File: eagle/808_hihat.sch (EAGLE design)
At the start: 101 parts, among them IC1 TL072P, IC3 TL071P, Q1 2N3904, Q10 2N3904, Q11 2N3904, Q12 2N3904, Q13 2N3906, Q14 2N3906, Q2 2N3904, Q3 2N3904, Q4 2N3904, Q5 2N3904, Q6 2N3904, Q7 2N3904, Q8 2N3904, Q9 2N3904

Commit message: 94pct ar
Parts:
- R130*, R140*, R173*: device TR808clone:R-EU_0207/5V -> TR808clone:R-EU_0207/7
- R145*, R162*: device TR808clone:R-EU_0207/7 -> TR808clone:R-EU_0207/5V
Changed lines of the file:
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@@
 <part name="V362" library="supply1" deviceset="GND" device=""/>
 <part name="V363" library="supply1" deviceset="GND" device=""/>
-<part name="R130*" library="TR808clone" deviceset="R-EU_" device="0207/5V" value="10K"/>
+<part name="R130*" library="TR808clone" deviceset="R-EU_" device="0207/7" value="10K"/>
 <part name="V364" library="supply1" deviceset="GND" device=""/>
 <part name="C60*" library="TR808clone" deviceset="CPOL-EU" device="E2.5-5" value="10/16"/>
@@
 <part name="R136*" library="TR808clone" deviceset="R-EU_" device="0207/5V" value="100R"/>
 <part name="R141*" library="TR808clone" deviceset="R-EU_" device="0207/5V" value="33K"/>
-<part name="R173*" library="TR808clone" deviceset="R-EU_" device="0207/5V" value="330K"/>
+<part name="R173*" library="TR808clone" deviceset="R-EU_" device="0207/7" value="330K"/>
 <part name="C63*" library="TR808clone" deviceset="CPOL-EU" device="E2.5-5" value=".47/50"/>
 <part name="V374" library="supply1" deviceset="GND" device=""/>
@@
 <part name="V375" library="supply1" deviceset="GND" device=""/>
 <part name="V376" library="supply1" deviceset="GND" device=""/>
-<part name="R145*" library="TR808clone" deviceset="R-EU_" device="0207/7" value="100R"/>
+<part name="R145*" library="TR808clone" deviceset="R-EU_" device="0207/5V" value="100R"/>
 <part name="R152*" library="TR808clone" deviceset="R-EU_" device="0207/5V" value="100R"/>
 <part name="R150*" library="TR808clone" deviceset="R-EU_" device="0207/5V" value="2M"/>
@@
 <part name="C74*" library="TR808clone" deviceset="C-EU" device="050-025X075" value="470p"/>
 <part name="R160*" library="TR808clone" deviceset="R-EU_" device="0207/5V" value="39K"/>
-<part name="R162*" library="TR808clone" deviceset="R-EU_" device="0207/7" value="33K"/>
+<part name="R162*" library="TR808clone" deviceset="R-EU_" device="0207/5V" value="33K"/>
 <part name="R158*" library="TR808clone" deviceset="R-EU_" device="0207/5V" value="47K"/>
 <part name="R157*" library="TR808clone" deviceset="R-EU_" device="0207/5V" value="47K"/>
@@
 <part name="R172*" library="TR808clone" deviceset="R-EU_" device="0207/7" value="1K"/>
 <part name="R132*" library="TR808clone" deviceset="R-EU_" device="0207/5V" value="100K"/>
-<part name="R140*" library="TR808clone" deviceset="R-EU_" device="0207/5V" value="33K"/>
+<part name="R140*" library="TR808clone" deviceset="R-EU_" device="0207/7" value="33K"/>
 <part name="R156*" library="TR808clone" deviceset="R-EU_" device="0207/7" value="22K"/>
 <part name="R154*" library="TR808clone" deviceset="R-EU_" device="0207/5V" value="22K"/>

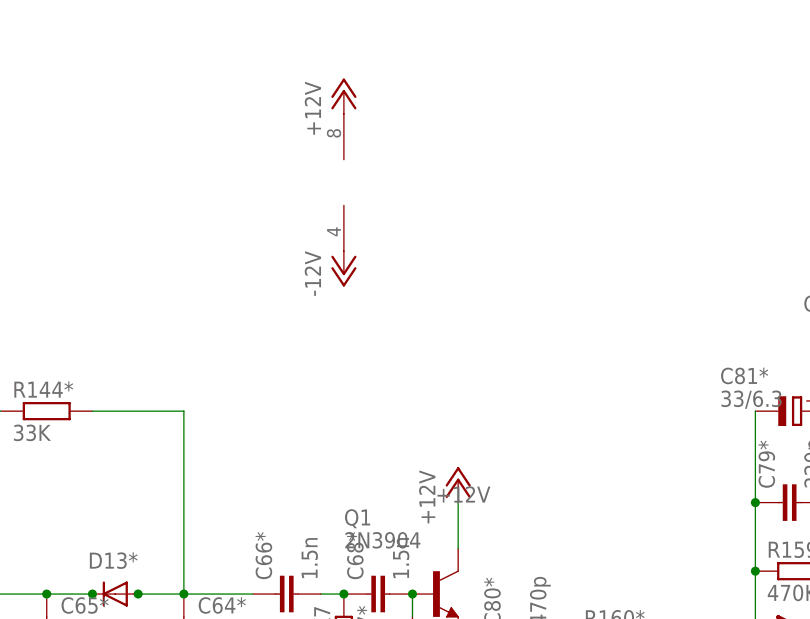
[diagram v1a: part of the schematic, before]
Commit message: 94pct6 ar
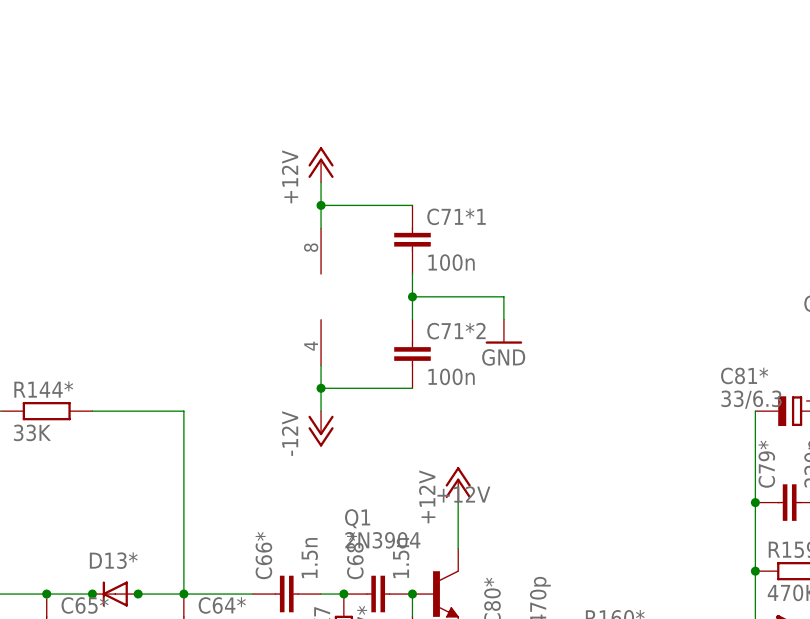
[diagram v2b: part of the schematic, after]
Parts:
- added C71*1, C71*2: 100n, TR808clone:C-EU3MM_PITCH
- C64*, C66*, C72*, C73*: device TR808clone:C-EU3.5MM_PITCH -> TR808clone:C-EU050-024X044
- C81*: device TR808clone:CPOL-EUE2-5 -> TR808clone:CPOL-EUE3.5-8
- R135*, R155*, R158*, R162*: device TR808clone:R-EU_0207/5V -> TR808clone:R-EU_0207/7
- R136*: device TR808clone:R-EU_0207/5V -> TR808clone:R-EU_0207/2V
- R156*, R172*: device TR808clone:R-EU_0207/7 -> TR808clone:R-EU_0207/5V
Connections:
- net +12V: now also C71*1.1
- net -12V: now also C71*2.2
- net GND: now also C71*1.2, C71*2.1
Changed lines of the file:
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@@
 <part name="R133*" library="TR808clone" deviceset="R-EU_" device="0207/7" value="10K"/>
 <part name="R134*" library="TR808clone" deviceset="R-EU_" device="0207/7" value="100K"/>
-<part name="R135*" library="TR808clone" deviceset="R-EU_" device="0207/5V" value="10K"/>
+<part name="R135*" library="TR808clone" deviceset="R-EU_" device="0207/7" value="10K"/>
 <part name="R137*" library="TR808clone" deviceset="R-EU_" device="0207/5V" value="470R"/>
 <part name="C62*" library="TR808clone" deviceset="CPOL-EU" device="E2.5-5" value=".47/50"/>
@@
 <part name="R143*" library="TR808clone" deviceset="R-EU_" device="0207/5V" value="33K"/>
 <part name="V371" library="supply1" deviceset="GND" device=""/>
-<part name="R136*" library="TR808clone" deviceset="R-EU_" device="0207/5V" value="100R"/>
+<part name="R136*" library="TR808clone" deviceset="R-EU_" device="0207/2V" value="100R"/>
 <part name="R141*" library="TR808clone" deviceset="R-EU_" device="0207/5V" value="33K"/>
 <part name="R173*" library="TR808clone" deviceset="R-EU_" device="0207/7" value="330K"/>
@@
 <part name="C65*" library="TR808clone" deviceset="C-EU" device="3.5MM_PITCH" value="1.5n"/>
 <part name="C70*" library="TR808clone" deviceset="C-EU" device="3.5MM_PITCH" value="1.5n"/>
-<part name="C64*" library="TR808clone" deviceset="C-EU" device="3.5MM_PITCH" value="1.5n"/>
+<part name="C64*" library="TR808clone" deviceset="C-EU" device="050-024X044" value="1.5n"/>
 <part name="C69*" library="TR808clone" deviceset="C-EU" device="3.5MM_PITCH" value="1.5n"/>
 <part name="V379" library="supply1" deviceset="GND" device=""/>
@@
 <part name="V381" library="supply1" deviceset="GND" device=""/>
 <part name="V382" library="supply1" deviceset="GND" device=""/>
-<part name="C66*" library="TR808clone" deviceset="C-EU" device="3.5MM_PITCH" value="1.5n"/>
-<part name="C72*" library="TR808clone" deviceset="C-EU" device="3.5MM_PITCH" value="1n"/>
+<part name="C66*" library="TR808clone" deviceset="C-EU" device="050-024X044" value="1.5n"/>
+<part name="C72*" library="TR808clone" deviceset="C-EU" device="050-024X044" value="1n"/>
 <part name="C68*" library="TR808clone" deviceset="C-EU" device="050-024X044" value="1.5n"/>
-<part name="C73*" library="TR808clone" deviceset="C-EU" device="3.5MM_PITCH" value="1n"/>
+<part name="C73*" library="TR808clone" deviceset="C-EU" device="050-024X044" value="1n"/>
 <part name="R147*" library="TR808clone" deviceset="R-EU_" device="0207/7" value="2K7"/>
 <part name="R153*" library="rcl" deviceset="R-US_" device="0207/5V" value="2K7"/>
 <part name="R146*" library="TR808clone" deviceset="R-EU_" device="0207/7" value="68K"/>
-<part name="R155*" library="TR808clone" deviceset="R-EU_" device="0207/5V" value="68K"/>
+<part name="R155*" library="TR808clone" deviceset="R-EU_" device="0207/7" value="68K"/>
 <part name="V383" library="supply1" deviceset="GND" device=""/>
 <part name="V384" library="supply1" deviceset="GND" device=""/>
@@
 <part name="C74*" library="TR808clone" deviceset="C-EU" device="050-025X075" value="470p"/>
 <part name="R160*" library="TR808clone" deviceset="R-EU_" device="0207/5V" value="39K"/>
-<part name="R162*" library="TR808clone" deviceset="R-EU_" device="0207/5V" value="33K"/>
-<part name="R158*" library="TR808clone" deviceset="R-EU_" device="0207/5V" value="47K"/>
+<part name="R162*" library="TR808clone" deviceset="R-EU_" device="0207/7" value="33K"/>
+<part name="R158*" library="TR808clone" deviceset="R-EU_" device="0207/7" value="47K"/>
 <part name="R157*" library="TR808clone" deviceset="R-EU_" device="0207/5V" value="47K"/>
 <part name="V389" library="supply1" deviceset="GND" device=""/>
 <part name="V390" library="supply1" deviceset="GND" device=""/>
 <part name="R159*" library="TR808clone" deviceset="R-EU_" device="0207/2V" value="470K"/>
-<part name="C81*" library="TR808clone" deviceset="CPOL-EU" device="E2-5" value="33/6.3"/>
+<part name="C81*" library="TR808clone" deviceset="CPOL-EU" device="E3.5-8" value="33/6.3"/>
 <part name="C79*" library="TR808clone" deviceset="C-EU" device="025-025X050" value="220p"/>
 <part name="R169*" library="TR808clone" deviceset="R-EU_" device="0207/7" value="1K"/>
@@
 <part name="C83*" library="TR808clone" deviceset="CPOL-EU" device="E2-5" value="33/6.3"/>
 <part name="C82*" library="TR808clone" deviceset="C-EU" device="025-025X050" value="220p"/>
-<part name="R172*" library="TR808clone" deviceset="R-EU_" device="0207/7" value="1K"/>
+<part name="R172*" library="TR808clone" deviceset="R-EU_" device="0207/5V" value="1K"/>
 <part name="R132*" library="TR808clone" deviceset="R-EU_" device="0207/5V" value="100K"/>
 <part name="R140*" library="TR808clone" deviceset="R-EU_" device="0207/7" value="33K"/>
-<part name="R156*" library="TR808clone" deviceset="R-EU_" device="0207/7" value="22K"/>
+<part name="R156*" library="TR808clone" deviceset="R-EU_" device="0207/5V" value="22K"/>
 <part name="R154*" library="TR808clone" deviceset="R-EU_" device="0207/5V" value="22K"/>
 <part name="R144*" library="TR808clone" deviceset="R-EU_" device="0207/5V" value="33K"/>
@@
 <part name="P+13" library="supply1" deviceset="+12V" device=""/>
 <part name="P-6" library="supply1" deviceset="-12V" device=""/>
+<part name="C71*1" library="TR808clone" deviceset="C-EU" device="3MM_PITCH" value="100n"/>
+<part name="C71*2" library="TR808clone" deviceset="C-EU" device="3MM_PITCH" value="100n"/>
+<part name="V5" library="supply1" deviceset="GND" device=""/>
 </parts>
 <sheets>
@@
 <instance part="Q13" gate="G$1" x="-50.8" y="93.98"/>
 <instance part="Q14" gate="G$1" x="-48.26" y="5.08"/>
-<instance part="IC1" gate="P" x="93.98" y="101.6"/>
-<instance part="P+5" gate="1" x="93.98" y="111.76"/>
-<instance part="P-5" gate="1" x="93.98" y="91.44"/>
+<instance part="IC1" gate="P" x="91.44" y="88.9"/>
+<instance part="P+5" gate="1" x="91.44" y="104.14"/>
+<instance part="P-5" gate="1" x="91.44" y="73.66"/>
 <instance part="IC3" gate="A" x="27.94" y="-30.48" rot="MR180"/>
 <instance part="P+13" gate="1" x="33.02" y="-38.1"/>
 <instance part="P-6" gate="1" x="22.86" y="-22.86"/>
+<instance part="C71*1" gate="G$1" x="101.6" y="96.52"/>
+<instance part="C71*2" gate="G$1" x="101.6" y="83.82"/>
+<instance part="V5" gate="1" x="111.76" y="83.82"/>
 </instances>
 <busses>
@@
 <pinref part="Q11" gate="G1" pin="E"/>
 </segment>
+<segment>
+<pinref part="V5" gate="1" pin="GND"/>
+<wire x1="111.76" y1="86.36" x2="111.76" y2="88.9" width="0.1524" layer="91"/>
+<pinref part="C71*2" gate="G$1" pin="1"/>
+<pinref part="C71*1" gate="G$1" pin="2"/>
+<wire x1="101.6" y1="86.36" x2="101.6" y2="88.9" width="0.1524" layer="91"/>
+<wire x1="101.6" y1="88.9" x2="101.6" y2="91.44" width="0.1524" layer="91"/>
+<wire x1="111.76" y1="88.9" x2="101.6" y2="88.9" width="0.1524" layer="91"/>
+<junction x="101.6" y="88.9"/>
+</segment>
 </net>
 <net name="N$219" class="0">
@@
 <pinref part="IC1" gate="P" pin="V+"/>
 <pinref part="P+5" gate="1" pin="+12V"/>
+<wire x1="91.44" y1="96.52" x2="91.44" y2="99.06" width="0.1524" layer="91"/>
+<pinref part="C71*1" gate="G$1" pin="1"/>
+<wire x1="91.44" y1="99.06" x2="91.44" y2="101.6" width="0.1524" layer="91"/>
+<wire x1="101.6" y1="99.06" x2="91.44" y2="99.06" width="0.1524" layer="91"/>
+<junction x="91.44" y="99.06"/>
 </segment>
 <segment>
@@
 <pinref part="IC1" gate="P" pin="V-"/>
 <pinref part="P-5" gate="1" pin="-12V"/>
-</segment>
-<segment>
+<wire x1="91.44" y1="76.2" x2="91.44" y2="78.74" width="0.1524" layer="91"/>
+<pinref part="C71*2" gate="G$1" pin="2"/>
+<wire x1="91.44" y1="78.74" x2="91.44" y2="81.28" width="0.1524" layer="91"/>
+<wire x1="101.6" y1="78.74" x2="91.44" y2="78.74" width="0.1524" layer="91"/>
+<junction x="91.44" y="78.74"/>
+</segment>
+<segment>

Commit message: rotated output amp looks promising
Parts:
- C68*: device TR808clone:C-EU050-024X044 -> TR808clone:C-EU050-025X075
- C69*, C80*: device TR808clone:C-EU3.5MM_PITCH -> TR808clone:C-EU050-024X044
- C71*1: device TR808clone:C-EU3MM_PITCH -> TR808clone:C-EU050-024X044
- R136*, R58*1: device TR808clone:R-EU_0207/2V -> TR808clone:R-EU_0207/5V
- R142*: device TR808clone:R-EU_0207/7 -> TR808clone:R-EU_0207/5V
- R147*: device TR808clone:R-EU_0207/7 -> TR808clone:R-EU_0309/10
- R156*, R157*, R160*: device TR808clone:R-EU_0207/5V -> TR808clone:R-EU_0207/7
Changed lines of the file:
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@@
 <part name="R143*" library="TR808clone" deviceset="R-EU_" device="0207/5V" value="33K"/>
 <part name="V371" library="supply1" deviceset="GND" device=""/>
-<part name="R136*" library="TR808clone" deviceset="R-EU_" device="0207/2V" value="100R"/>
+<part name="R136*" library="TR808clone" deviceset="R-EU_" device="0207/5V" value="100R"/>
 <part name="R141*" library="TR808clone" deviceset="R-EU_" device="0207/5V" value="33K"/>
 <part name="R173*" library="TR808clone" deviceset="R-EU_" device="0207/7" value="330K"/>
@@
 <part name="C70*" library="TR808clone" deviceset="C-EU" device="3.5MM_PITCH" value="1.5n"/>
 <part name="C64*" library="TR808clone" deviceset="C-EU" device="050-024X044" value="1.5n"/>
-<part name="C69*" library="TR808clone" deviceset="C-EU" device="3.5MM_PITCH" value="1.5n"/>
+<part name="C69*" library="TR808clone" deviceset="C-EU" device="050-024X044" value="1.5n"/>
 <part name="V379" library="supply1" deviceset="GND" device=""/>
 <part name="V380" library="supply1" deviceset="GND" device=""/>
@@
 <part name="C66*" library="TR808clone" deviceset="C-EU" device="050-024X044" value="1.5n"/>
 <part name="C72*" library="TR808clone" deviceset="C-EU" device="050-024X044" value="1n"/>
-<part name="C68*" library="TR808clone" deviceset="C-EU" device="050-024X044" value="1.5n"/>
+<part name="C68*" library="TR808clone" deviceset="C-EU" device="050-025X075" value="1.5n"/>
 <part name="C73*" library="TR808clone" deviceset="C-EU" device="050-024X044" value="1n"/>
-<part name="R147*" library="TR808clone" deviceset="R-EU_" device="0207/7" value="2K7"/>
+<part name="R147*" library="TR808clone" deviceset="R-EU_" device="0309/10" value="2K7"/>
 <part name="R153*" library="rcl" deviceset="R-US_" device="0207/5V" value="2K7"/>
 <part name="R146*" library="TR808clone" deviceset="R-EU_" device="0207/7" value="68K"/>
@@
 <part name="V383" library="supply1" deviceset="GND" device=""/>
 <part name="V384" library="supply1" deviceset="GND" device=""/>
-<part name="C80*" library="TR808clone" deviceset="C-EU" device="3.5MM_PITCH" value="470p"/>
+<part name="C80*" library="TR808clone" deviceset="C-EU" device="050-024X044" value="470p"/>
 <part name="C74*" library="TR808clone" deviceset="C-EU" device="050-025X075" value="470p"/>
-<part name="R160*" library="TR808clone" deviceset="R-EU_" device="0207/5V" value="39K"/>
+<part name="R160*" library="TR808clone" deviceset="R-EU_" device="0207/7" value="39K"/>
 <part name="R162*" library="TR808clone" deviceset="R-EU_" device="0207/7" value="33K"/>
 <part name="R158*" library="TR808clone" deviceset="R-EU_" device="0207/7" value="47K"/>
-<part name="R157*" library="TR808clone" deviceset="R-EU_" device="0207/5V" value="47K"/>
+<part name="R157*" library="TR808clone" deviceset="R-EU_" device="0207/7" value="47K"/>
 <part name="V389" library="supply1" deviceset="GND" device=""/>
 <part name="V390" library="supply1" deviceset="GND" device=""/>
@@
 <part name="R132*" library="TR808clone" deviceset="R-EU_" device="0207/5V" value="100K"/>
 <part name="R140*" library="TR808clone" deviceset="R-EU_" device="0207/7" value="33K"/>
-<part name="R156*" library="TR808clone" deviceset="R-EU_" device="0207/5V" value="22K"/>
+<part name="R156*" library="TR808clone" deviceset="R-EU_" device="0207/7" value="22K"/>
 <part name="R154*" library="TR808clone" deviceset="R-EU_" device="0207/5V" value="22K"/>
 <part name="R144*" library="TR808clone" deviceset="R-EU_" device="0207/5V" value="33K"/>
@@
 <part name="OH_LEVEL" library="pot" deviceset="3RP/1610N" device="" value="100KA"/>
 <part name="DECAY" library="pot" deviceset="3RP/1610N" device="" value="2MB"/>
-<part name="R142*" library="TR808clone" deviceset="R-EU_" device="0207/7" value="33K"/>
+<part name="R142*" library="TR808clone" deviceset="R-EU_" device="0207/5V" value="33K"/>
 <part name="V44" library="supply1" deviceset="GND" device=""/>
 <part name="V45" library="supply1" deviceset="GND" device=""/>
@@
 <part name="V3" library="supply1" deviceset="GND" device=""/>
 <part name="R59*1" library="TR808clone" deviceset="R-EU_" device="0207/5V" value="82K"/>
-<part name="R58*1" library="TR808clone" deviceset="R-EU_" device="0207/2V" value="560R"/>
+<part name="R58*1" library="TR808clone" deviceset="R-EU_" device="0207/5V" value="560R"/>
 <part name="IC1" library="linear" deviceset="TL072" device="P"/>
 <part name="U$1" library="eurorack" deviceset="POWER" device=""/>
@@
 <part name="P+13" library="supply1" deviceset="+12V" device=""/>
 <part name="P-6" library="supply1" deviceset="-12V" device=""/>
-<part name="C71*1" library="TR808clone" deviceset="C-EU" device="3MM_PITCH" value="100n"/>
+<part name="C71*1" library="TR808clone" deviceset="C-EU" device="050-024X044" value="100n"/>
 <part name="C71*2" library="TR808clone" deviceset="C-EU" device="3MM_PITCH" value="100n"/>
 <part name="V5" library="supply1" deviceset="GND" device=""/>

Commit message: routed
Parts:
- R59*1: device TR808clone:R-EU_0207/5V -> TR808clone:R-EU_0207/7
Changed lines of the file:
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@@
 <part name="C16*1" library="TR808clone" deviceset="C-EU" device="3.5MM_PITCH" value="3.3n"/>
 <part name="V3" library="supply1" deviceset="GND" device=""/>
-<part name="R59*1" library="TR808clone" deviceset="R-EU_" device="0207/5V" value="82K"/>
+<part name="R59*1" library="TR808clone" deviceset="R-EU_" device="0207/7" value="82K"/>
 <part name="R58*1" library="TR808clone" deviceset="R-EU_" device="0207/5V" value="560R"/>
 <part name="IC1" library="linear" deviceset="TL072" device="P"/>
